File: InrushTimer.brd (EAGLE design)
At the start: 62.2 x 36 mm, 71 parts, among them IC1 TLC272D, IC2 555, IC3 4076N, Q2 TRANSISTOR-FET_2N7002, Q3 TRANSISTOR-FET_2N7002, Q4 TRANSISTOR-FET_2N7002, Q5 TRANSISTOR-FET_2N7002, Q6 DIODES_ZTX451DIODES_ZTX451_0_0, T1 MMBTA05, U1 ROHM_BY_ELEMENT14_BATCH_1_BU4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

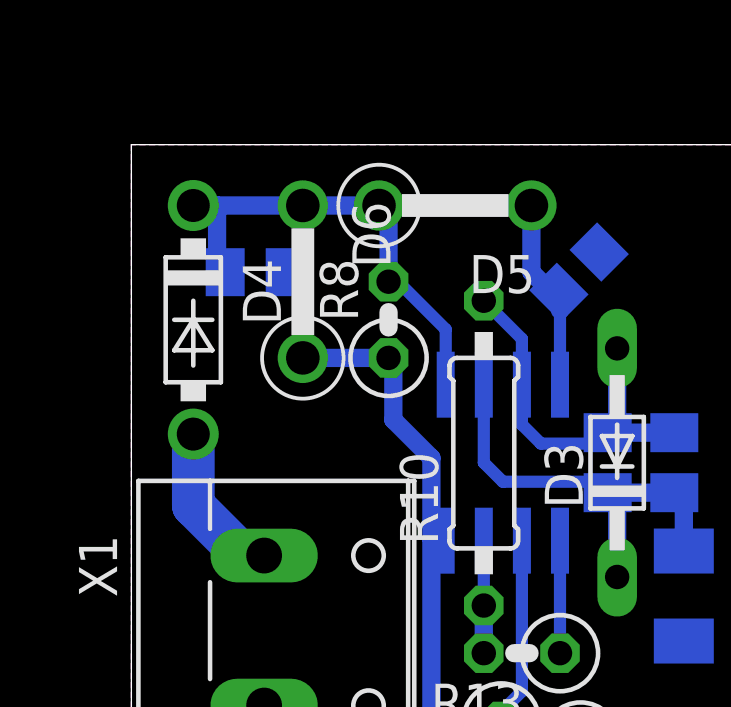
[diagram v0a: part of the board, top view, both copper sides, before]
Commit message: Layout changes.
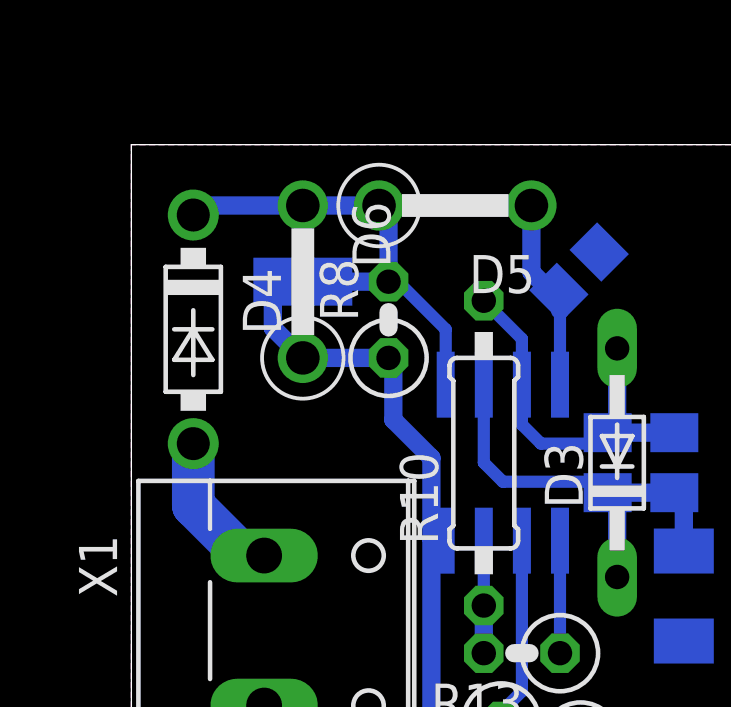
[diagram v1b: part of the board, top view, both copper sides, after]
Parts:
- moved C5 1.62 mm to (5.71, 31.4), turned to 180 degrees
- moved D4 0.32 mm to (2.06, 29.8)
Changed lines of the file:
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@@
 <setting verticaltext="up"/>
 </settings>
-<grid distance="0.05" unitdist="inch" unit="inch" style="lines" multiple="1" display="yes" altdistance="0.00625" altunitdist="inch" altunit="inch"/>
+<grid distance="0.05" unitdist="inch" unit="inch" style="lines" multiple="1" display="yes" altdistance="0.0125" altunitdist="inch" altunit="inch"/>
 <layers>
 <layer number="1" name="Top" color="4" fill="1" visible="yes" active="yes"/>
@@
 <element name="R3" library="rcl" package="0207/2V" value="10K" x="18.0975" y="9.8425" rot="R225"/>
 <element name="C10" library="rcl" package="C0805K" value="10pF (DNF)" x="73.025" y="27.305" rot="MR180"/>
-<element name="D4" library="diode" package="DO41-7.6" value="STTH110" x="2.06375" y="30.1625" rot="R270"/>
+<element name="D4" library="diode" package="DO41-7.6" value="STTH110" x="2.06375" y="29.845" rot="R270"/>
 <element name="IC1" library="linear" package="SO08" value="TLC272D" x="12.3825" y="25.4" smashed="yes" rot="MR0">
 <attribute name="NAME" x="15.0495" y="23.495" size="1.27" layer="26" rot="MR90"/>
@@
 <attribute name="MF" value="" x="56.515" y="30.7975" size="1.778" layer="27" rot="R90" display="off"/>
 </element>
-<element name="C5" library="rcl" package="C0805K" value="10nF" x="4.1275" y="31.75" rot="MR0"/>
+<element name="C5" library="rcl" package="C0805K" value="10nF" x="5.715" y="31.4325" rot="MR180"/>
 <element name="C4" library="rcl" package="C050-024X044" value="10nF" x="20.6375" y="8.255" rot="R45"/>
 <element name="C6" library="rcl" package="C0805K" value="1nF" x="18.0975" y="25.4" rot="MR90"/>
@@
 <wire x1="70.00875" y1="18.415" x2="72.920721875" y2="17.090525" width="0" layer="19" extent="1-1"/>
 <wire x1="45.24375" y1="1.74625" x2="70.00875" y2="8.255" width="0" layer="19" extent="1-1"/>
-<wire x1="41.165" y1="12.065" x2="45.24375" y2="1.74625" width="0" layer="19" extent="16-16"/>
-<wire x1="38.735" y1="9.525" x2="41.165" y2="12.065" width="0" layer="19" extent="16-16"/>
+<wire x1="38.735" y1="9.525" x2="45.24375" y2="1.74625" width="0" layer="19" extent="1-1"/>
+<wire x1="41.165" y1="12.065" x2="38.735" y2="9.525" width="0" layer="19" extent="16-16"/>
 <wire x1="32.86125" y1="16.98625" x2="38.735" y2="9.525" width="0" layer="19" extent="1-1"/>
 <wire x1="24.710525" y1="9.153025" x2="32.86125" y2="16.98625" width="0" layer="19" extent="1-1"/>
@@
 <wire x1="15.5575" y1="5.08" x2="15.5575" y2="5.395" width="0.4064" layer="16"/>
 <wire x1="17.2593" y1="3.7973" x2="17.2593" y2="5.08" width="0.4064" layer="16"/>
-<wire x1="5.1275" y1="31.75" x2="5.715" y2="31.1625" width="0.6096" layer="16"/>
-<wire x1="5.715" y1="31.1625" x2="5.715" y2="28.8925" width="0.6096" layer="16"/>
 <wire x1="5.715" y1="28.8925" x2="8.5725" y2="28.8925" width="0.6096" layer="16"/>
 <wire x1="18.995525" y1="10.740525" x2="19.25855" y2="10.4775" width="0.6096" layer="16"/>
@@
 <wire x1="10.00125" y1="22.86" x2="10.00125" y2="14.976971875" width="0.6096" layer="16"/>
 <wire x1="10.00125" y1="14.976971875" x2="10.531971875" y2="14.976971875" width="0.6096" layer="16"/>
+<wire x1="5.715" y1="28.8925" x2="5.6675" y2="28.8925" width="0.6096" layer="16"/>
+<wire x1="5.715" y1="28.8925" x2="4.715" y2="29.8925" width="0.6096" layer="16"/>
+<wire x1="4.715" y1="29.8925" x2="4.715" y2="31.4325" width="0.6096" layer="16"/>
 <wire x1="83.65" y1="32.7" x2="81.11" y2="35.24" width="0" layer="19" extent="1-1"/>
 <wire x1="77.62875" y1="26.035" x2="83.65" y2="32.7" width="0" layer="19" extent="1-1"/>
@@
 <wire x1="45.24375" y1="6.82625" x2="45.87875" y2="9.04875" width="0" layer="19" extent="1-1"/>
 <wire x1="33.765" y1="12.065" x2="42.79125" y2="14.12875" width="0" layer="19" extent="16-16"/>
+<wire x1="32.385" y1="14.605" x2="33.765" y2="12.065" width="0" layer="19" extent="16-16"/>
 <wire x1="34.501434375" y1="6.84706875" x2="33.765" y2="12.065" width="0" layer="19" extent="16-16"/>
 <wire x1="30.7975" y1="3.81" x2="34.501434375" y2="6.84706875" width="0" layer="19" extent="16-16"/>
 <wire x1="19.25855" y1="10.4775" x2="18.415" y2="5.08" width="0" layer="19" extent="16-16"/>
-<wire x1="32.385" y1="14.605" x2="33.765" y2="12.065" width="0" layer="19" extent="16-16"/>
 <wire x1="12.065" y1="11.43" x2="15.5575" y2="5.395" width="0" layer="19" extent="16-16"/>
 <wire x1="15.594253125" y1="32.42175" x2="8.73125" y2="28.73375" width="0" layer="19" extent="16-16"/>
@@
 <contactref element="IC1" pad="5"/>
 <contactref element="R8" pad="2"/>
-<wire x1="2.06375" y1="33.9725" x2="2.8575" y2="33.9725" width="0.6096" layer="16"/>
-<wire x1="2.8575" y1="33.9725" x2="5.715" y2="33.9725" width="0.6096" layer="16"/>
-<wire x1="3.1275" y1="31.75" x2="2.8575" y2="32.02" width="0.6096" layer="16"/>
-<wire x1="2.8575" y1="32.02" x2="2.8575" y2="33.9725" width="0.6096" layer="16"/>
+<wire x1="2.06375" y1="33.9725" x2="5.715" y2="33.9725" width="0.6096" layer="16"/>
 <wire x1="5.715" y1="33.9725" x2="8.255" y2="33.9725" width="0.6096" layer="16"/>
 <wire x1="8.5725" y1="31.4325" x2="8.5725" y2="33.9725" width="0.6096" layer="16"/>
@@
 <wire x1="8.89" y1="31.4325" x2="8.5725" y2="31.4325" width="0.4064" layer="16"/>
 <wire x1="10.4775" y1="28" x2="10.4775" y2="29.845" width="0.4064" layer="16"/>
+<wire x1="2.06375" y1="33.9725" x2="2.06375" y2="33.655" width="0.6096" layer="16"/>
+<wire x1="8.5725" y1="31.4325" x2="6.715" y2="31.4325" width="0.6096" layer="16"/>
 </signal>
 <signal name="N$7">
@@
 <wire x1="41.165" y1="14.605" x2="45.79125" y2="14.12875" width="0" layer="19" extent="16-16"/>
 <wire x1="41.165" y1="13.335" x2="41.165" y2="14.605" width="0" layer="19" extent="16-16"/>
-<wire x1="35.2425" y1="26.035" x2="45.79125" y2="14.12875" width="0" layer="19" extent="16-16"/>
+<wire x1="35.2425" y1="26.035" x2="41.165" y2="14.605" width="0" layer="19" extent="16-16"/>
 </signal>
 <signal name="ON_B">
@@
 <wire x1="4.425" y1="22.30375" x2="3.73125" y2="22.30375" width="1.4224" layer="16"/>
 <wire x1="3.73125" y1="22.30375" x2="2.06375" y2="23.97125" width="1.4224" layer="16"/>
-<wire x1="2.06375" y1="23.97125" x2="2.06375" y2="26.3525" width="1.4224" layer="16"/>
+<wire x1="2.06375" y1="23.97125" x2="2.06375" y2="26.035" width="1.4224" layer="16"/>
 </signal>
 <signal name="ON_A_SYNC">
